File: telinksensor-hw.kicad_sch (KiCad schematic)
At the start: 81 parts, among them J1 ANT, J2 3W RTD, J3 Conn_01x05, J4 RTD 2W, Q1 2N7002, SW1 SW_Push, U1 TLSR8258, U2 SHT40, U3 BMP390, Y1 24MHz

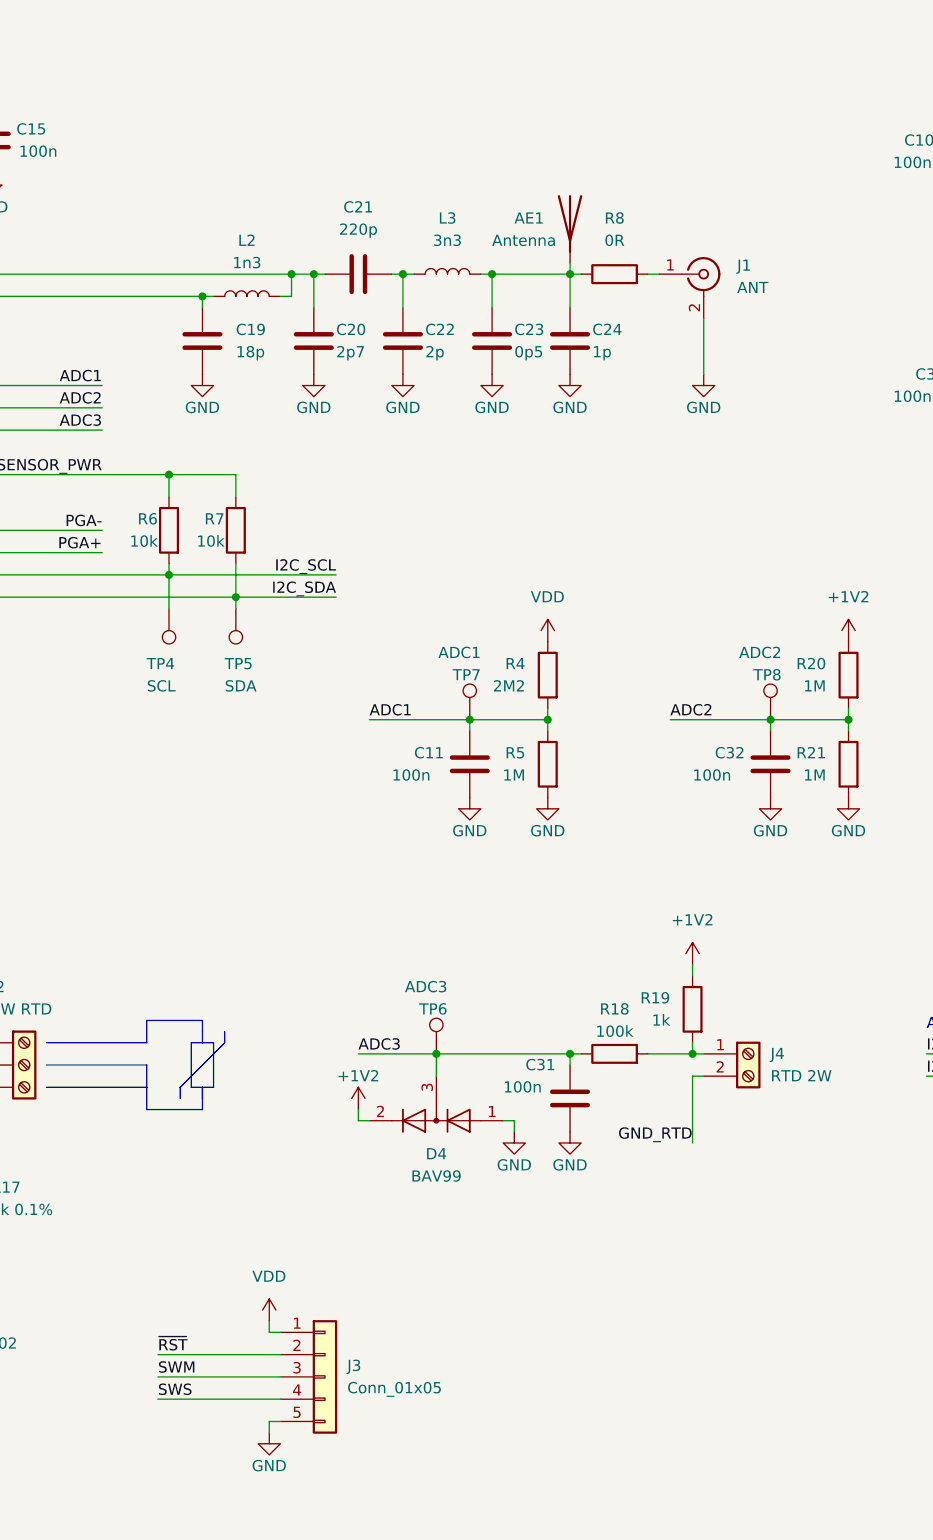
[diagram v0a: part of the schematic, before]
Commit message: Outline done
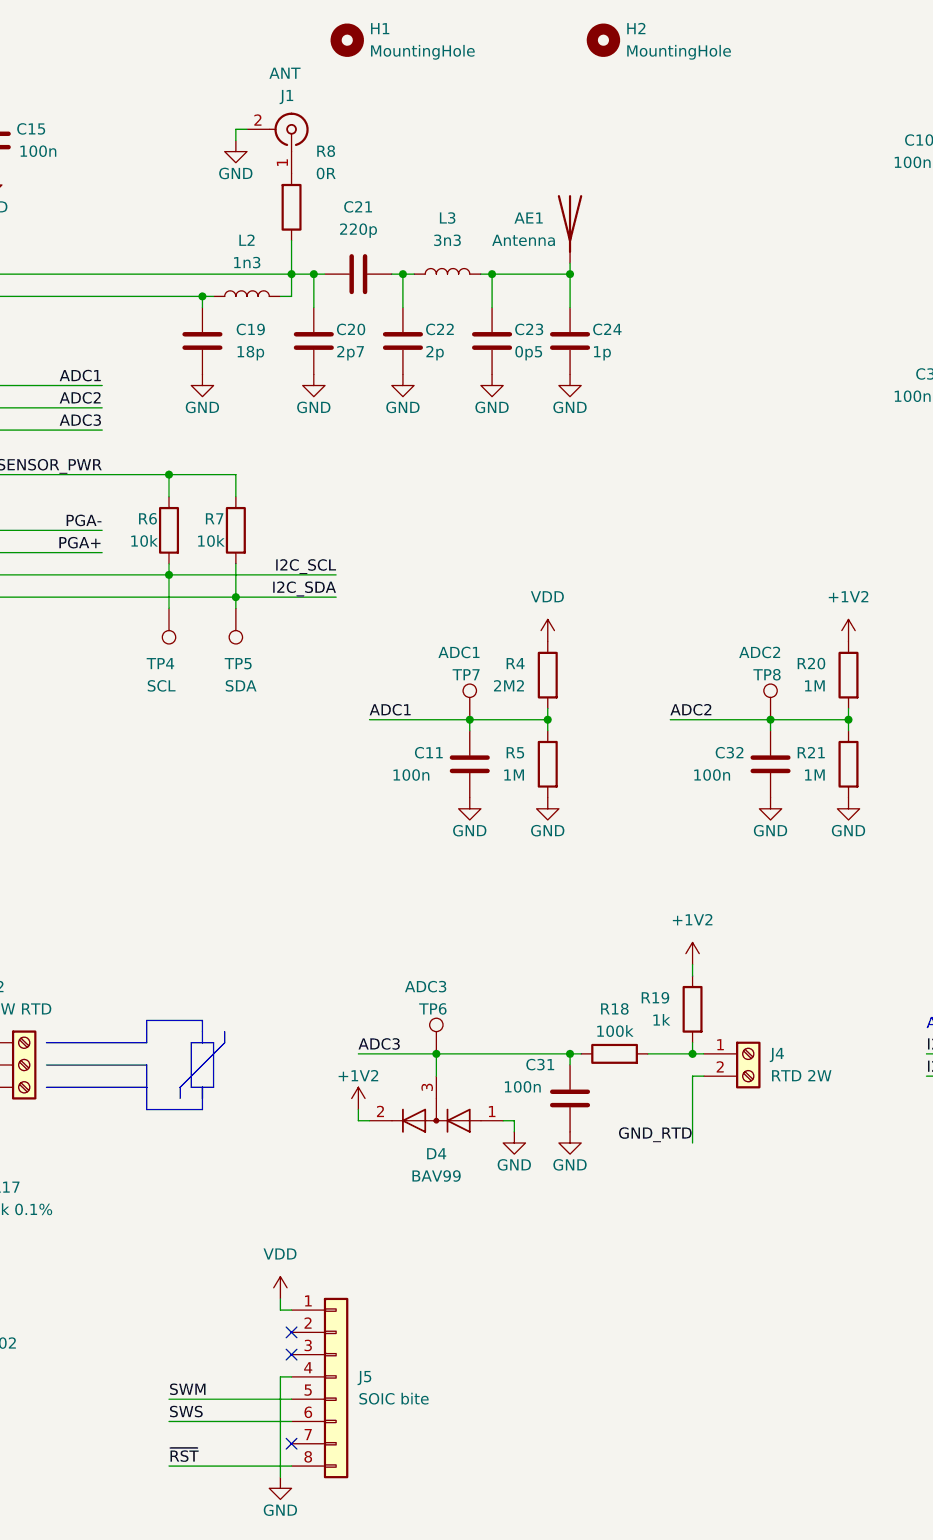
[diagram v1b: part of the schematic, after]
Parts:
- removed J3: Conn_01x05, symbol Connector_Generic:Conn_01x05
- added H1, H2: MountingHole, MountingHole:MountingHole_3.2mm_M3_Pad_Via, symbol Mechanical:MountingHole
- added J5: SOIC bite, soicbite:SOIC_clipProgSmall, symbol Connector_Generic:Conn_01x08
- AE1: footprint (none) -> RF_Antenna:Johanson_2450AT18x100
- C19, C20, C21, C22, C23, C24: footprint Capacitor_SMD:C_0603_1608Metric -> Capacitor_SMD:C_0402_1005Metric
- J1: footprint (none) -> Connector_Coaxial:U.FL_Molex_MCRF_73412-0110_Vertical
- J2: footprint (none) -> TerminalBlock:TerminalBlock_bornier-3_P5.08mm
- J4: footprint (none) -> TerminalBlock:TerminalBlock_bornier-2_P5.08mm
- L1: footprint (none) -> Inductor_SMD:L_0805_2012Metric
- L2, L3: footprint Inductor_SMD:L_0603_1608Metric -> Inductor_SMD:L_0402_1005Metric
- R8: footprint Resistor_SMD:R_0603_1608Metric -> Resistor_SMD:R_0402_1005Metric
- SW1: footprint (none) -> Button_Switch_SMD:SW_SPST_EVQPE1
- TP1, TP10, TP2, TP3, TP4, TP5, TP6, TP7, TP8, TP9: footprint TestPoint:TestPoint_Pad_1.5x1.5mm -> TestPoint:TestPoint_Pad_D1.0mm
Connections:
- net GND: now also J5.4 (Pin_4)
- net SWM: now also J5.5 (Pin_5)
- net SWS: now also J5.6 (Pin_6)
- net VDD: now also J5.1 (Pin_1)
- net ~{RST}: now also J5.8 (Pin_8)
- net at AE1.1 (A), C23.1, C24.1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: no longer R8.1
- net at C20.1, C21.1, L2.2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: now also R8.1
- no-connect marks 6 -> 9
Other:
- moved on the sheet: J1
